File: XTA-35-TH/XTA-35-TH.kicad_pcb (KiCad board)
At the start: 4 copper layers, 222.1 x 98.7 mm, 27 parts, among them J1 XTA_Connector, U4 RPI_PICO

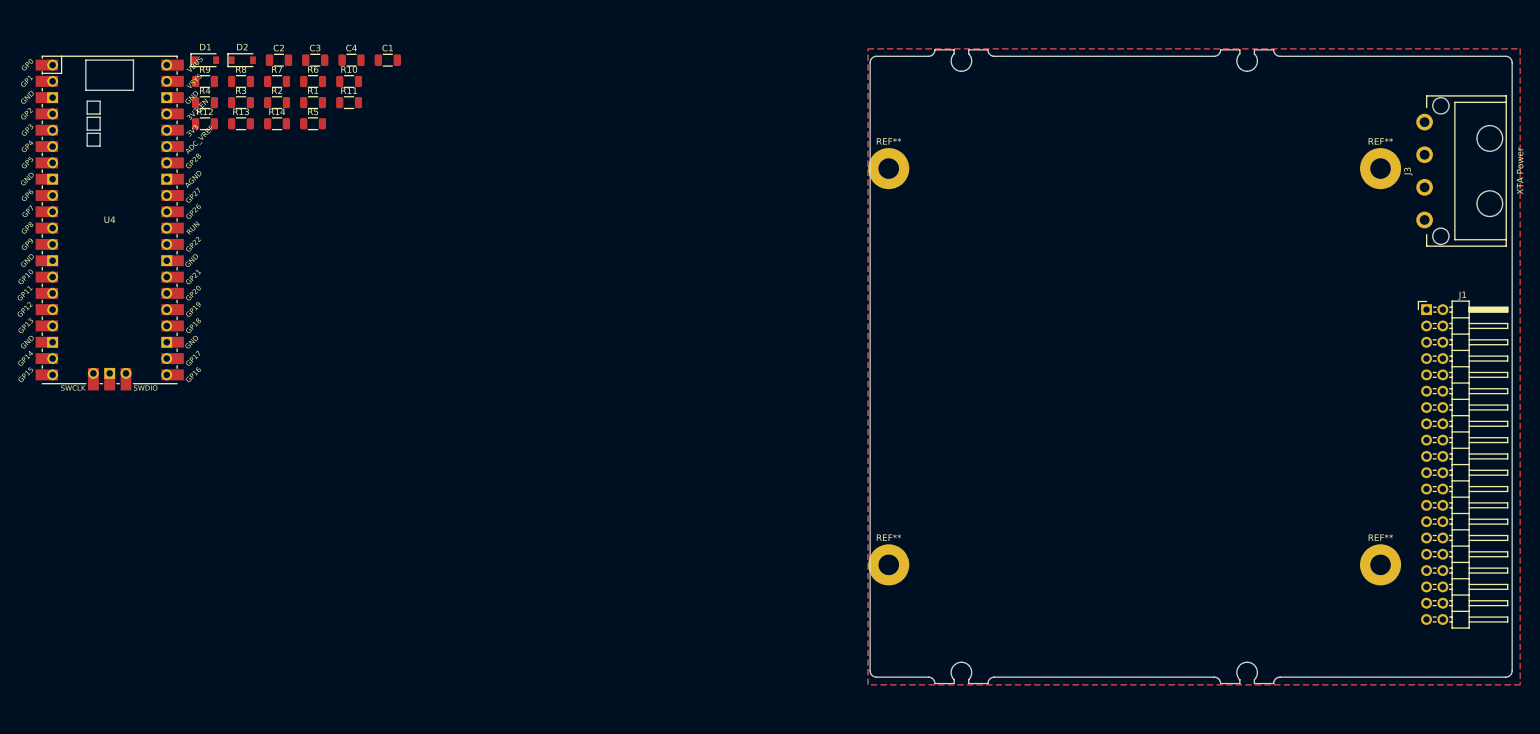
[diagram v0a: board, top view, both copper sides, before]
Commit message: Misc board work.
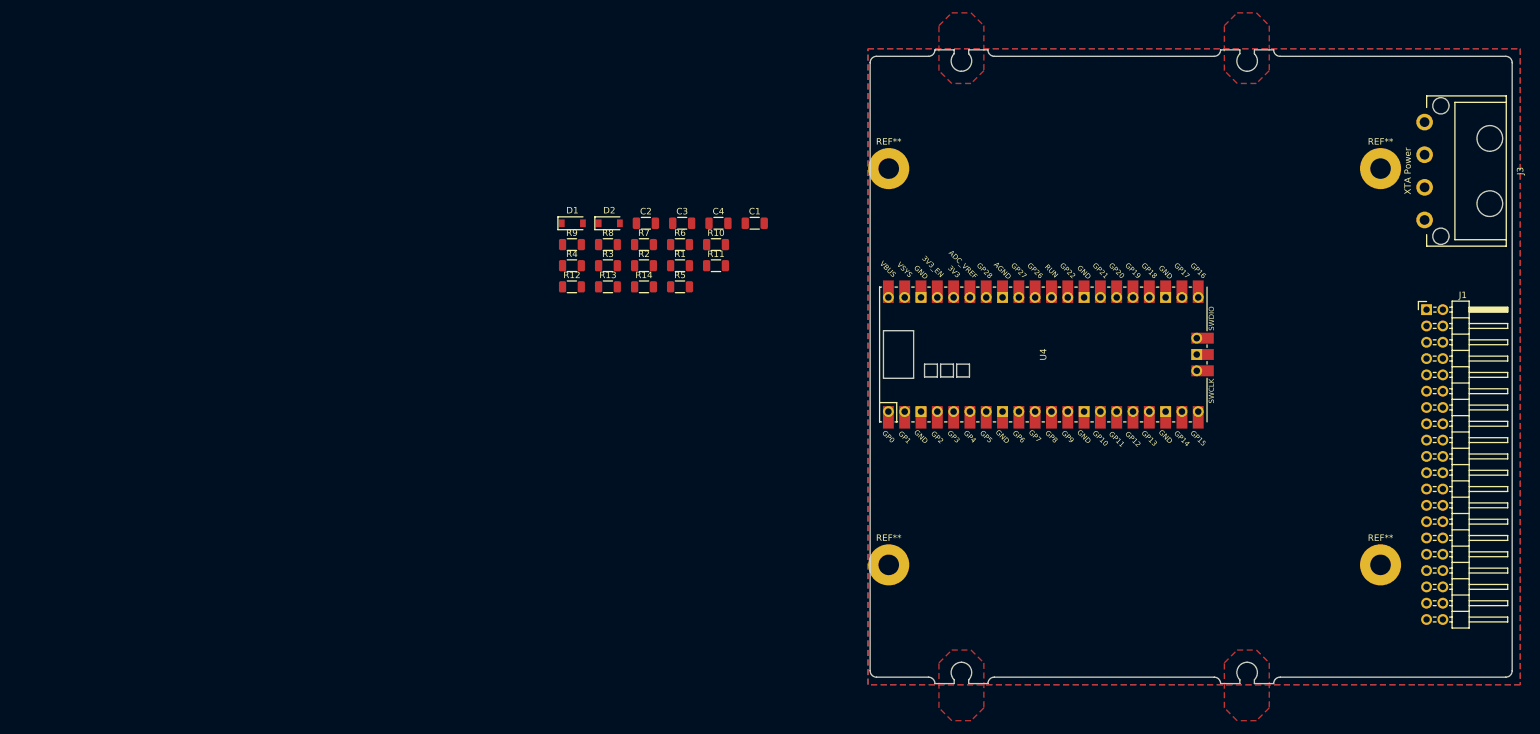
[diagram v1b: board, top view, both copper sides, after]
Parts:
- J3: renamed from XTA Power; value J3 -> XTA Power
- moved U4 146.9 mm to (177.2, 78.1), turned to 90 degrees
- moved C1 62.5 mm to (132.2, 57.7)
- moved C3 62.5 mm to (120.9, 57.7)
- moved R10 62.5 mm to (126.2, 61.0)
- moved R11 62.5 mm to (126.2, 64.3)
- moved C2 62.5 mm to (115.3, 57.7)
- moved D1 62.5 mm to (103.8, 57.7)
- moved D2 62.5 mm to (109.6, 57.7)
- moved R1 62.5 mm to (120.6, 64.3)
- moved R12 62.5 mm to (103.7, 67.6)
- moved R13 62.5 mm to (109.4, 67.6)
- moved R14 62.5 mm to (115.0, 67.6)
- moved R2 62.5 mm to (115.0, 64.3)
- moved R3 62.5 mm to (109.4, 64.3)
- moved R4 62.5 mm to (103.7, 64.3)
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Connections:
- J3 pad 1: (no net) -> Net-(J3-Pad1)
- J3 pad 2: (no net) -> GND
- J3 pad 3: (no net) -> GND
- J3 pad 4: (no net) -> IBM_5V_POWER
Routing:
- added copper zone on F.Cu, net (none)
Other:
- board size 222.1 x 98.7 mm -> 100 x 98.7 mm
